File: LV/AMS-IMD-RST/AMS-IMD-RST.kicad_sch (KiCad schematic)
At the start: 53 parts, among them J1 2P Droit 2-11-2022, J2 2P Droit 2-11-2022, J3 2P Droit 2-11-2022, J4 2P Droit 2-11-2022, J5 2P Droit 2-11-2022, J7 4P Droit 22-11-2042, K1 Relais PCB, K2 Bistable V23079B1201B301, K3 Relais PCB, K4 Bistable V23079B1201B301, Q1 NMOS SQ2348ES-T1_GE3, Q2 NMOS SQ2348ES-T1_GE3, Q3 NMOS SQ2348ES-T1_GE3, Q4 NMOS SQ2348ES-T1_GE3, Q5 NMOS SQ2348ES-T1_GE3, Q6 NMOS SQ2348ES-T1_GE3, U1 Alim LP TSR_0.5-2450, U2 ${SIM.PARAMS}, U3 LM358, U4 LM397, U5 LM397, U6 LM358

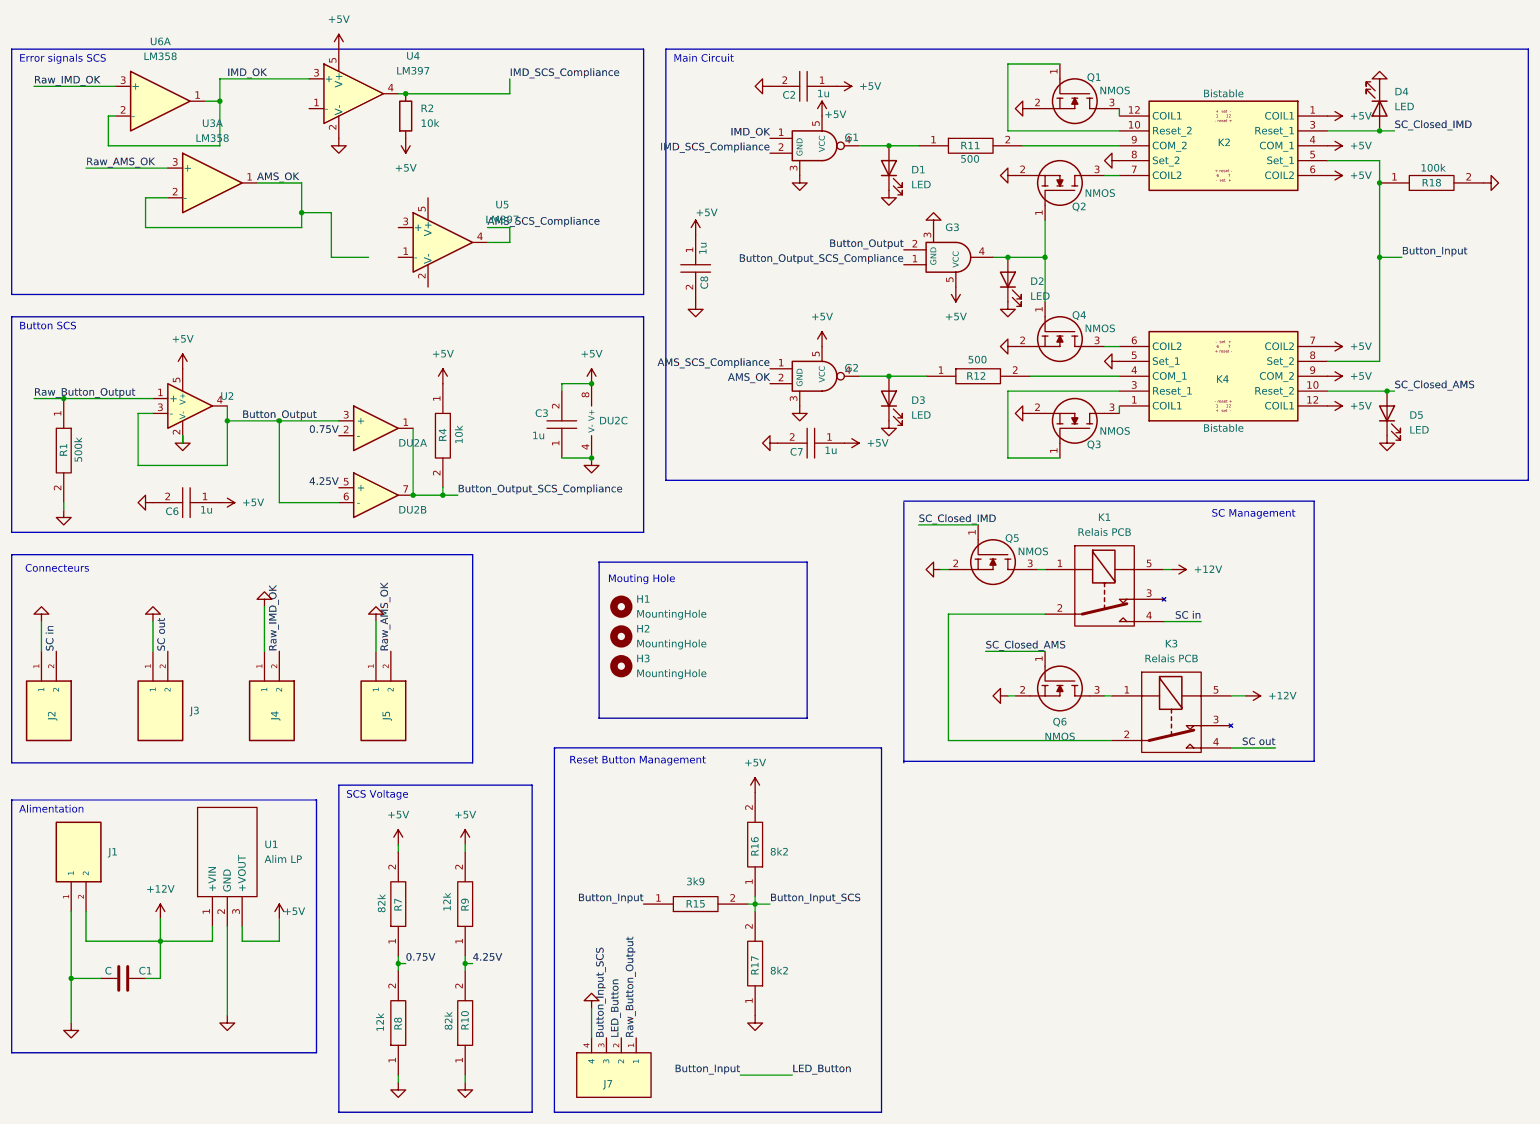
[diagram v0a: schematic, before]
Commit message: SCS added
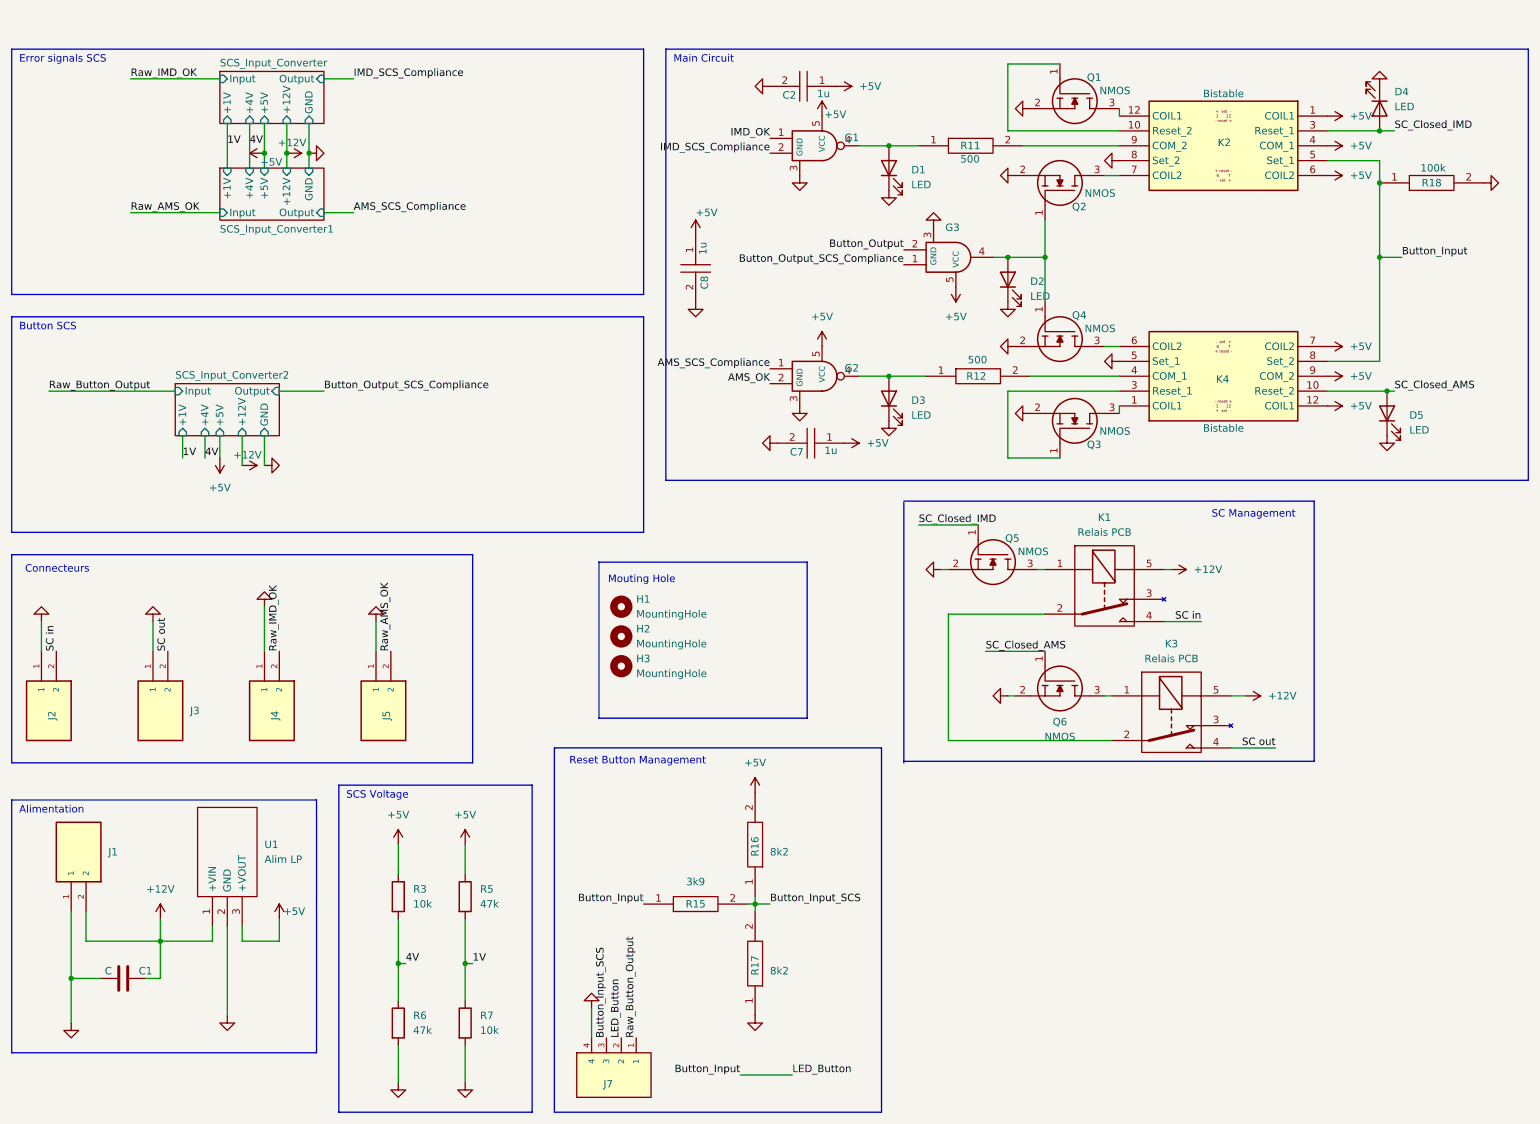
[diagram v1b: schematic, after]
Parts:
- removed C3, C6: 1u, EPSA_lib:CAPC2012X130N, symbol EPSA_Lib:Condensateur 0805Y1000104JXT
- removed DU2: Opamp_Dual, Package_SO:TSSOP-8_4.4x3mm_P0.65mm, symbol EPSA_Lib:Comparator_Dual
- removed R1: 500k, EPSA_lib:RESC3216X70N, symbol EPSA_Lib:Résistance RK73H2BLTDD2152F
- removed R10, R7: 82k, EPSA_lib:RESC3216X70N, symbol EPSA_Lib:Résistance RK73H2BLTDD2152F
- removed R2: 10k, symbol Device:R
- removed R4: 10k, EPSA_lib:RESC3216X70N, symbol EPSA_Lib:Résistance RK73H2BLTDD2152F
- removed R8, R9: 12k, EPSA_lib:RESC3216X70N, symbol EPSA_Lib:Résistance RK73H2BLTDD2152F
- removed U2: ${SIM.PARAMS}, Package_TO_SOT_SMD:SOT-353_SC-70-5_Handsoldering, symbol EPSA_Lib:Opamp
- removed U3, U6: LM358, symbol Amplifier_Operational:LM358
- removed U4, U5: LM397, Package_TO_SOT_SMD:SOT-23-5, symbol Comparator:LM397
- added R3, R7: 10k, symbol Device:R
- added R5, R6: 47k, symbol Device:R
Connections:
- net +5V: now also R3.1, R5.1
- net GND: now also R6.2, R7.2
- new net 1V: R5.2, R7.1
- new net 4V: R3.2, R6.1
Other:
- added sheet SCS_Input_Converter (${KIPRJMOD}/../scs_input_converter.kicad_sch)
- added sheet SCS_Input_Converter1 (${KIPRJMOD}/../scs_input_converter.kicad_sch)
- added sheet SCS_Input_Converter2 (${KIPRJMOD}/../scs_input_converter.kicad_sch)
